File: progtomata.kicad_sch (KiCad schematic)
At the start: 26 parts, among them P1 USB_C_Plug_USB2.0, SW1 SW_SPDT, U1 STM32F407VGTx, U2 AMS1117-3.3, Y1 8MHz

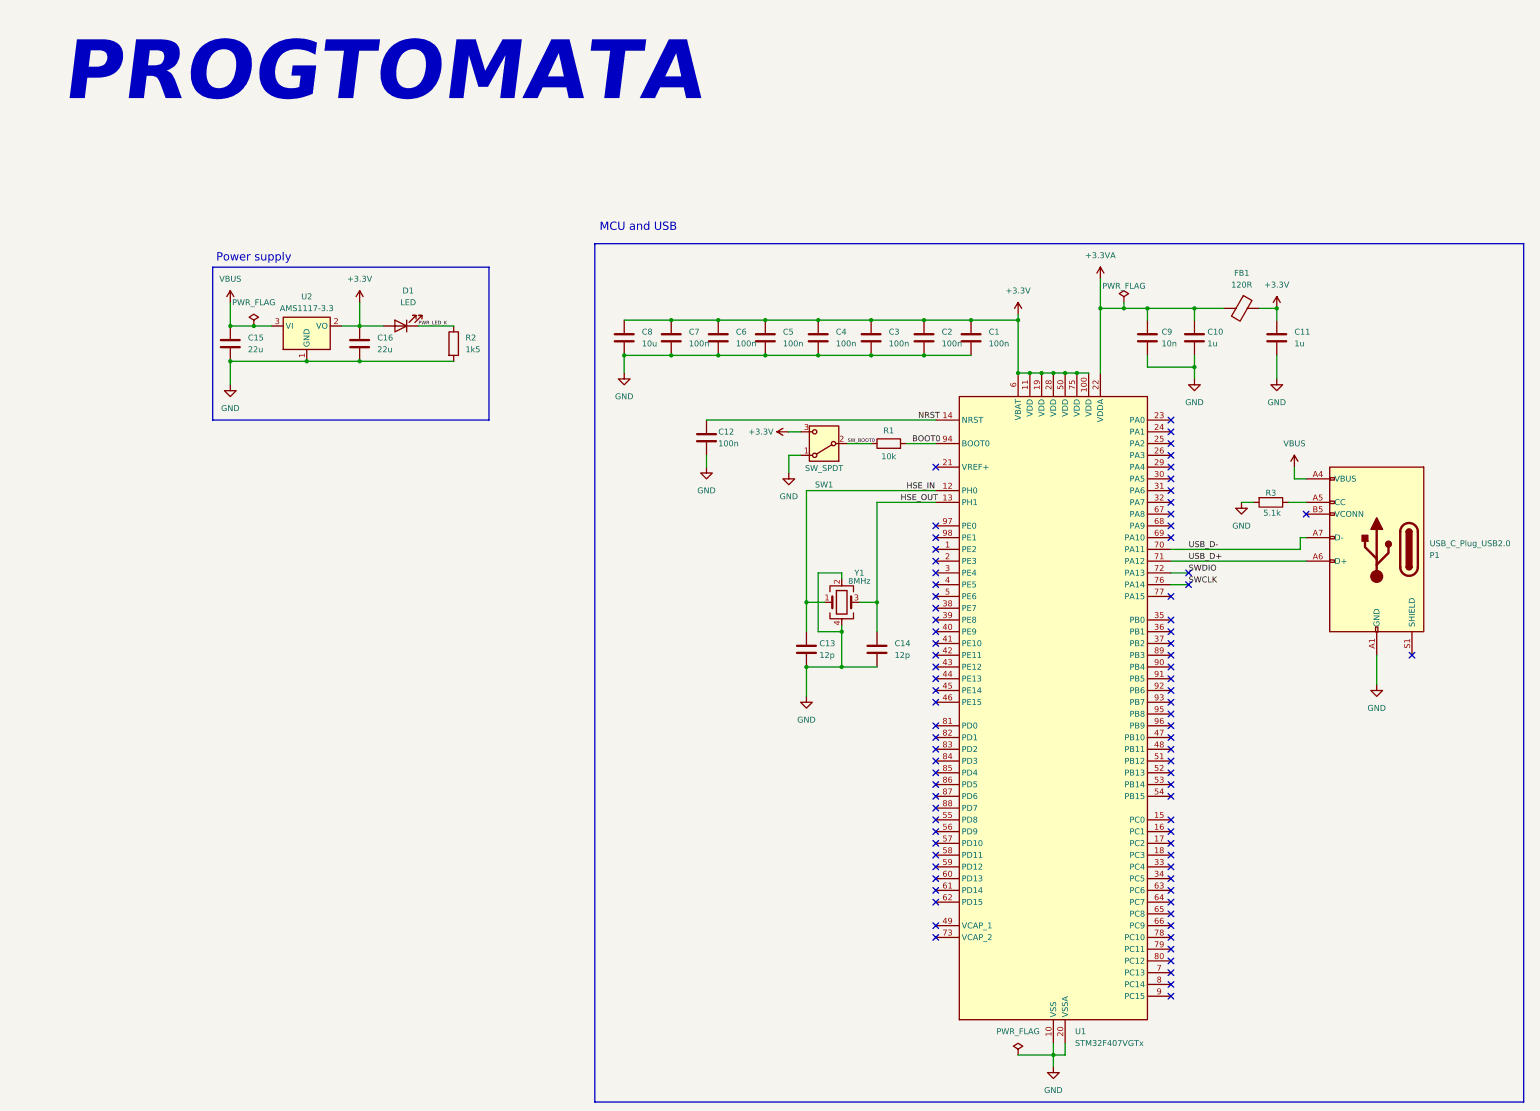
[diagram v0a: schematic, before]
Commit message: Update schematics
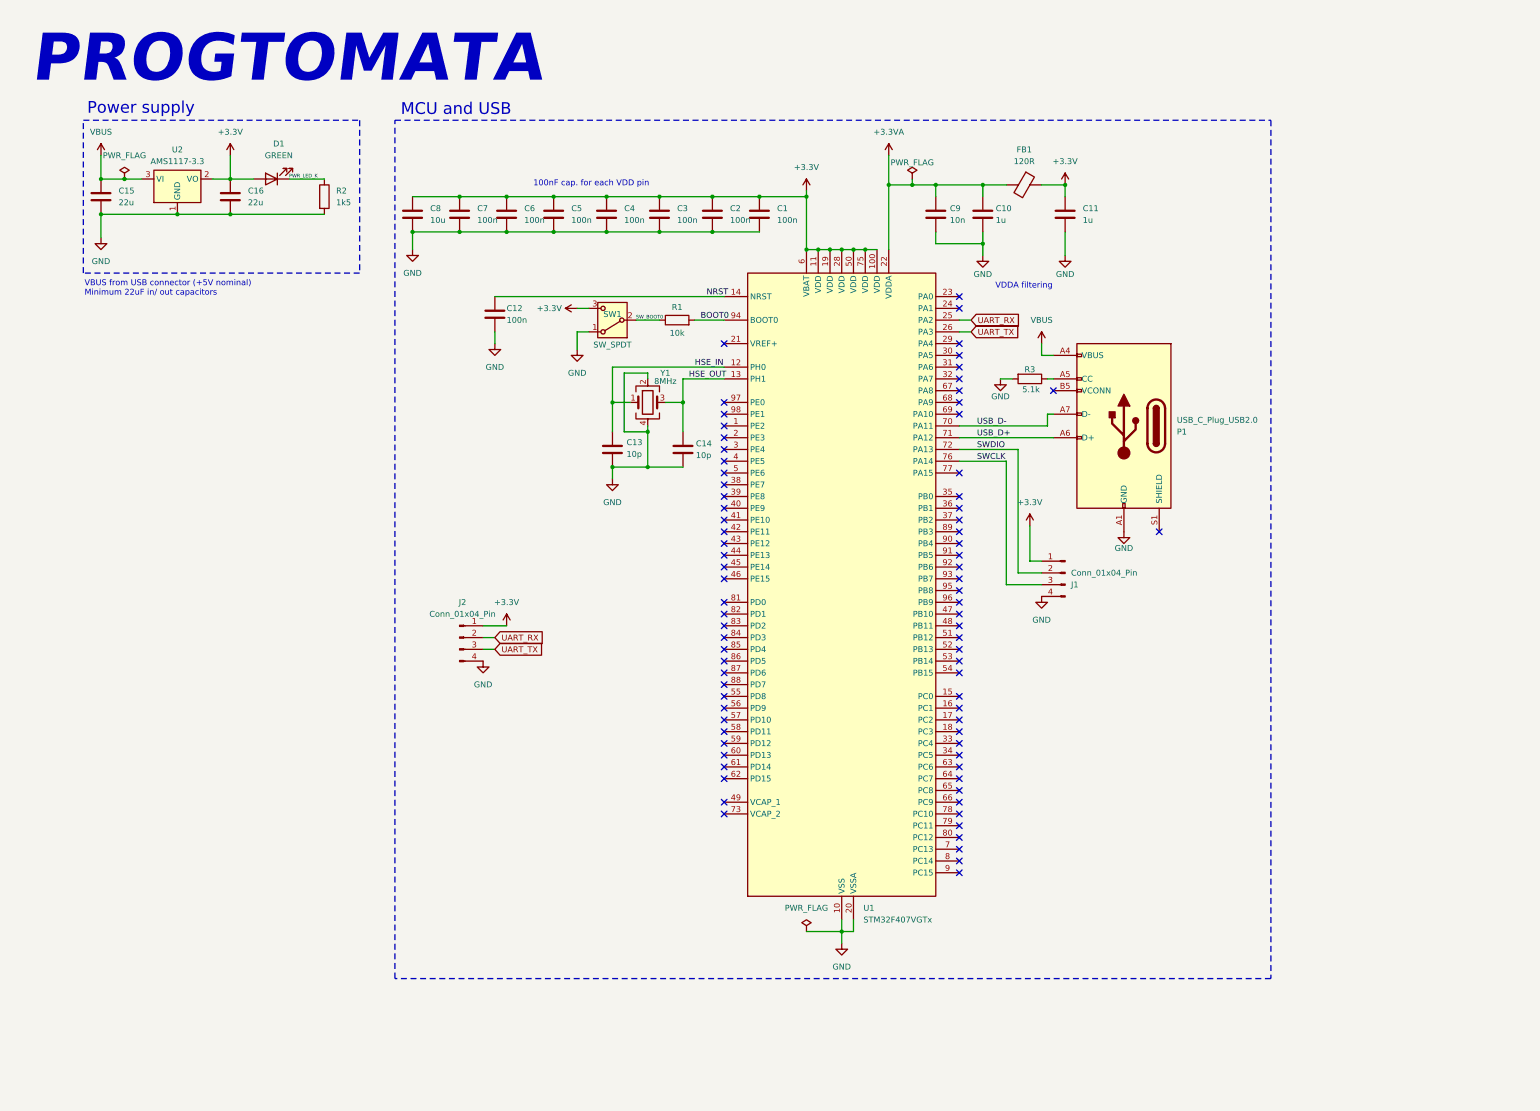
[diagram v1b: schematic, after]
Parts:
- added J1, J2: Conn_01x04_Pin, Connector_PinHeader_2.54mm:PinHeader_1x04_P2.54mm_Vertical, symbol Connector:Conn_01x04_Pin
- C1, C10, C11, C12, C2, C3, C4, C5, C6, C7, C9: footprint (none) -> Capacitor_SMD:C_0402_1005Metric
- C13, C14: value 12p -> 10p; footprint (none) -> Capacitor_SMD:C_0402_1005Metric
- C15, C16: footprint (none) -> Capacitor_SMD:C_0805_2012Metric
- C8: footprint (none) -> Capacitor_SMD:C_0603_1608Metric
- D1: value LED -> GREEN; footprint (none) -> LED_SMD:LED_0402_1005Metric
- FB1: footprint (none) -> Inductor_SMD:L_0603_1608Metric
- P1: footprint (none) -> Connector_USB:USB_C_Plug_Molex_105444
- R1, R2, R3: footprint (none) -> Resistor_SMD:R_0402_1005Metric
- SW1: footprint (none) -> Button_Switch_THT:SW_E-Switch_EG1224_SPDT_Angled
- Y1: footprint (none) -> Crystal:Crystal_SMD_3225-4Pin_3.2x2.5mm
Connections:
- net +3.3V: now also J1.1 (Pin_1), J2.1 (Pin_1)
- net GND: now also J1.4 (Pin_4), J2.4 (Pin_4)
- net SWCLK: now also J1.3 (Pin_3)
- net SWDIO: now also J1.2 (Pin_2)
- net UART_RX: now reaches U1.25 (PA2)
- net UART_RX: now also J2.2 (Pin_2)
- net UART_TX: now reaches U1.26 (PA3)
- net UART_TX: now also J2.3 (Pin_3)
- no-connect marks 83 -> 79
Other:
- note added: "100nF cap. for each VDD pin"
- note added: "VBUS from USB connector (+5V nominal) Minimum 22uF in/ out capacitors"
- note added: "VDDA filtering"
- moved on the sheet: C1, C10, C11, C12, C13, C14, C15, C16, C2, C3, C4, C5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
